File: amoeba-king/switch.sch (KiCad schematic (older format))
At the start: 2 parts

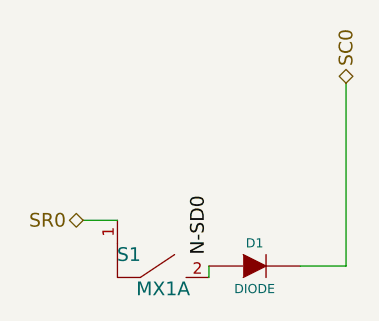
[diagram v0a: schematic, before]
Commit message: Getting ready for final review, before sending for production
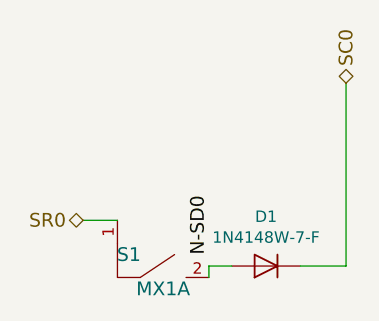
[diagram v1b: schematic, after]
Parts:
- removed D1: DIODE, Diode_SMD:D_0805_2012Metric_Pad1.15x1.40mm_HandSolder, symbol amoeba-royale-rescue:DIODE-amoeba-rescue
- added D1: 1N4148W-7-F, Diode_SMD:D_SOD-323, symbol Device:D
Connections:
- net SC0: now also D1.1 (K)
- net at S1.2: now also D1.2 (A)
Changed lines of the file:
@@
-	1    0    0    -1
-$EndComp
-$Comp
-L amoeba-royale-rescue:DIODE-amoeba-rescue D?
-U 1 1 55DBAE85
-P 5200 3550
-AR Path="/55DBAE85" Ref="D?"  Part="1"
-AR Path="/55D92FDB/55DBAE5B/55DBAE85" Ref="D1"  Part="1"
-F 0 "D1" H 5200 3650 40  0000 C CNN
-F 1 "DIODE" H 5200 3450 40  0000 C CNN
-F 2 "Diode_SMD:D_0805_2012Metric_Pad1.15x1.40mm_HandSolder" H 5200 3550 60  0001 C CNN
-F 3 "~" H 5200 3550 60  0000 C CNN
-	1    5200 3550
 	1    0    0    -1
 $EndComp
@@
 Text HLabel 4450 3350 0    60   BiDi ~ 0
 SR0
+$Comp
+L Device:D D1
+U 1 1 5EC43574
+P 5250 3550
+F 0 "D1" H 5250 3334 50  0000 C CNN
+F 1 "1N4148W-7-F" H 5250 3425 50  0000 C CNN
+F 2 "Diode_SMD:D_SOD-323" H 5250 3550 50  0001 C CNN
+F 3 "~" H 5250 3550 50  0001 C CNN
+	1    5250 3550
+	-1   0    0    1
+$EndComp
+Wire Wire Line
+	5100 3550 5000 3550
 $EndSCHEMATC

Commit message: Various Layout Improvements
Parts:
- D1: footprint Diode_SMD:D_SOD-323 -> Diode_SMD:D_SOD-123
- S1: symbol amoeba-royale-rescue:MX1A-amoeba-rescue -> amoeba-king-rescue:MX1A-amoeba-rescue-amoeba-royale-rescue
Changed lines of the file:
@@
 	5000 3550 5000 3600
 $Comp
-L amoeba-royale-rescue:MX1A-amoeba-rescue S?
+L amoeba-king-rescue:MX1A-amoeba-rescue-amoeba-royale-rescue S?
 U 1 1 55DBAE7F
 P 4800 3750
@@
 F 0 "D1" H 5250 3334 50  0000 C CNN
 F 1 "1N4148W-7-F" H 5250 3425 50  0000 C CNN
-F 2 "Diode_SMD:D_SOD-323" H 5250 3550 50  0001 C CNN
+F 2 "Diode_SMD:D_SOD-123" H 5250 3550 50  0001 C CNN
 F 3 "~" H 5250 3550 50  0001 C CNN
 	1    5250 3550
